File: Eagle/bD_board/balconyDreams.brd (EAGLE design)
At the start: 64.8 x 80 mm, 35 parts, among them IC1 7805L, Q1 2N7002, Q2 2N7002, Q3 2N7002, Q4 2N7002, Q5 2N7002, Q6 2N7002, Q7 2N7002, Q8 2N7002, U1 MKR1000, X2 MKDSN1,5/2-5,08

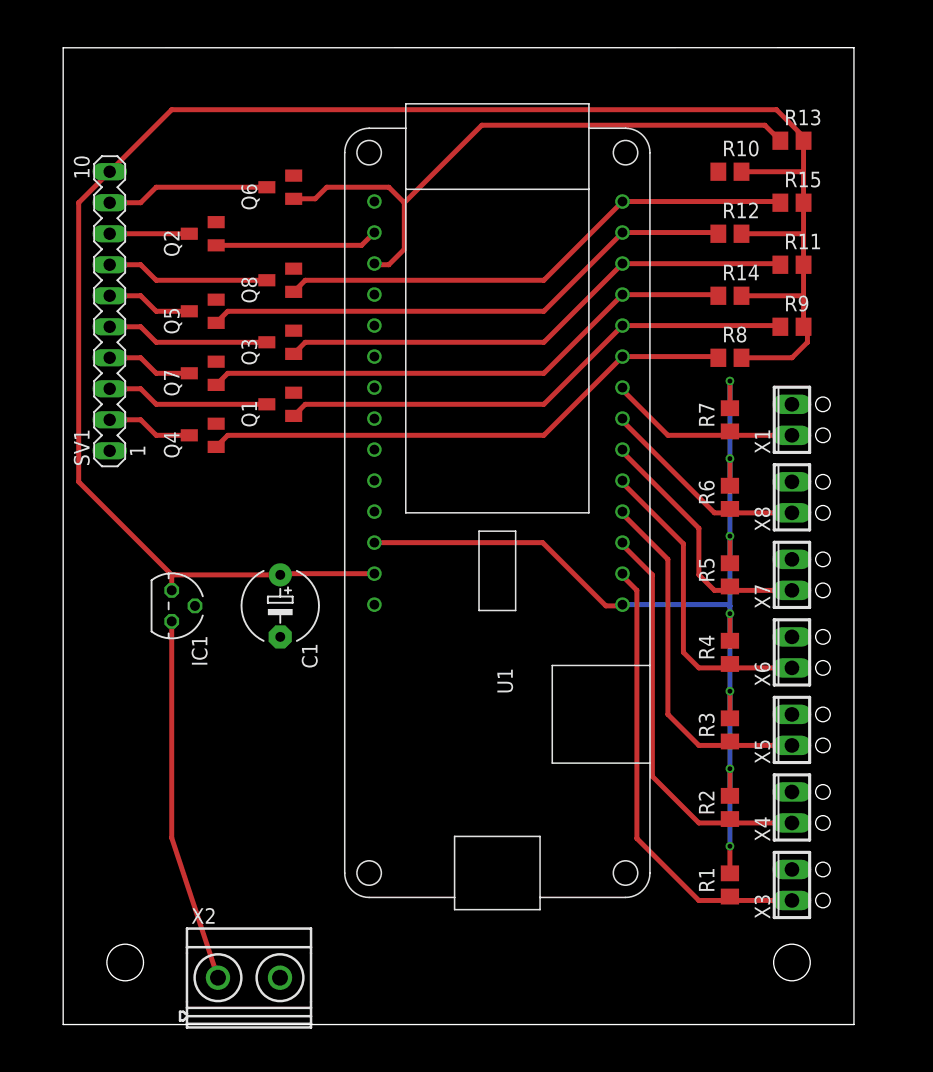
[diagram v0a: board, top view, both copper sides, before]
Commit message: Lots of stuff - ready for review
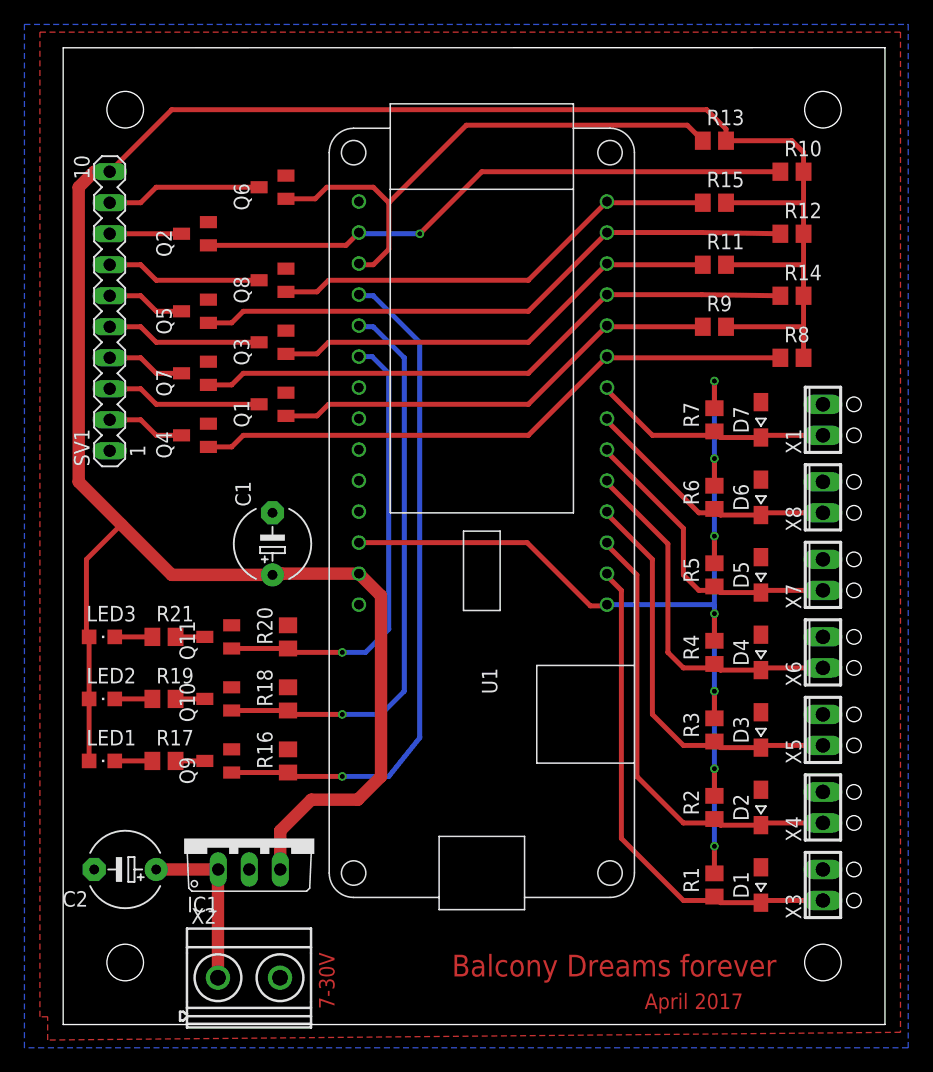
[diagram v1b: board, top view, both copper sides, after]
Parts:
- added C2: 0.33uF, rcl:E5-6
- added D1, D2, D3, D4, D5, D6, D7: (no value), diode:SOD323-W
- added LED1, LED2, LED3: (no value), led:CHIPLED_0805
- added Q10, Q11, Q9: 2N7002, transistors_gaui:SOT23
- added R16, R18, R20: 10k, rcl:R0805
- added R17, R19, R21: 330R, rcl:R0805
- C1: value (none) -> 1uF
- IC1: value 7805L -> 7805TV; device linear:TO92 -> linear:TO220V
- R10, R11, R12, R13, R14, R15, R8, R9: value (none) -> 10k
- moved IC1 20.1 mm to (15.2, 15.2), turned to 0 degrees
- moved R11 6.35 mm to (53.3, 62.2)
- moved R13 6.35 mm to (53.3, 72.4)
- moved R15 6.35 mm to (53.3, 67.3)
- moved R9 6.35 mm to (53.3, 57.1)
- moved C1 5.12 mm to (17.1, 39.4), turned to 90 degrees
- moved R10 5.08 mm to (59.7, 69.8)
- moved R12 5.08 mm to (59.7, 64.8)
- moved R14 5.08 mm to (59.7, 59.7)
- moved R8 5.08 mm to (59.7, 54.6)
- moved X1 2.54 mm to (62.2, 49.5)
- moved X3 2.54 mm to (62.2, 11.4)
- moved X4 2.54 mm to (62.2, 17.8)
- moved X5 2.54 mm to (62.2, 24.1)
- moved X6 2.54 mm to (62.2, 30.5)
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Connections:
- new net LED1: Q9.1, R16.1, U1.18
- new net LED2: Q10.1, R18.1, U1.19
- new net LED3: Q11.1, R20.1, U1.20
- new net N$1: LED1.C, R17.1
- new net N$2: Q9.3, R17.2
- new net N$3: Q10.3, R19.2
- new net N$4: LED2.C, R19.1
- new net N$5: Q11.3, R21.2
- new net N$6: LED3.C, R21.1
- net A0: now also D1.C
- net A1: now also D2.C
- net A2: now also D3.C
- net A3: now also D4.C
- net A4: now also D5.C
- net A5: now also D6.C
- net A6: now also D7.C
- net GND: now also C2.-, D1.A, D2.A, D3.A, D4.A, D5.A, D6.A, D7.A, Q10.2, Q11.2, Q9.2, R16.2, R18.2, R20.2
- net VCC: now also IC1.3, LED1.A, LED2.A, LED3.A; no longer IC1.1
- net V_INPUT: now also C2.+, IC1.1; no longer IC1.3
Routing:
- net LED1: track 0.00 -> 56.3 mm, vias 0 -> 1
- net VCC: track 153.1 -> 201.7 mm
- net LED2: track 0.00 -> 47.4 mm, vias 0 -> 1
- net LED3: track 0.00 -> 38.0 mm, vias 0 -> 1
- net RELAIS_7: track 13.4 -> 49.4 mm, vias 0 -> 1
- net V_INPUT: track 29.8 -> 14.0 mm
- net RELAIS_8: track 50.8 -> 45.0 mm
- net RELAIS_6: track 43.0 -> 37.3 mm
- net RELAIS_2: track 43.0 -> 37.3 mm
- net RELAIS_1: track 44.2 -> 50.0 mm
- net RELAIS_3: track 44.2 -> 49.9 mm
- net RELAIS_5: track 44.2 -> 49.9 mm
- net RELAIS_4: track 43.0 -> 37.3 mm
- net A1: track 33.4 -> 37.4 mm
- net A6: track 15.9 -> 19.8 mm
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- added copper zone on layer 1, net GND
- added copper zone on layer 16, net GND
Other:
- board size 64.8 x 80 mm -> 67.3 x 80 mm
- board text added: "7-30V"
- board text added: "April 2017"
- board text added: "Balcony Dreams forever"
